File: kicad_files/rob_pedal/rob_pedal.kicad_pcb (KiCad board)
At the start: 2 copper layers, 56.5 x 56.8 mm, 52 parts, among them J1 OD_IN, J2 ODR_OUT, J3 9V, J4 SHO_IN, J5 SHO_OUT, Q1 BS170, Q2 BS170, Q3 BS170, Q4 BS170

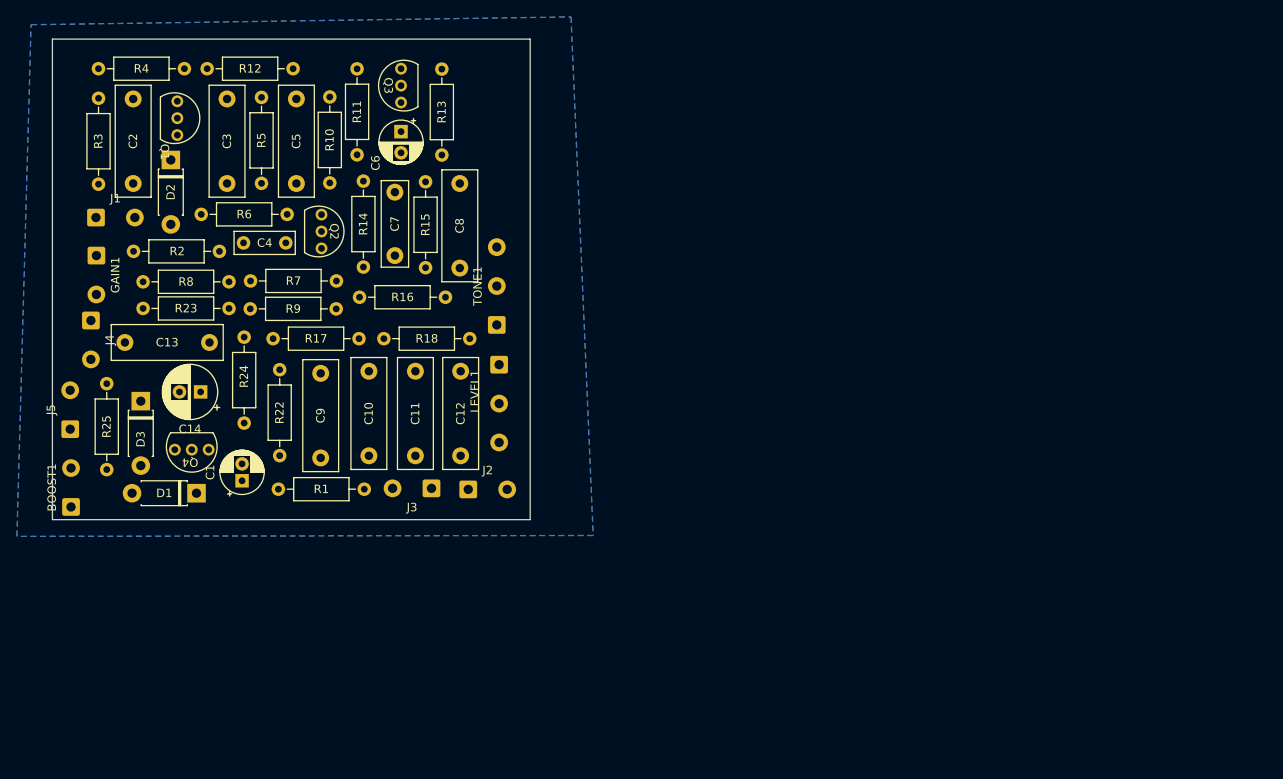
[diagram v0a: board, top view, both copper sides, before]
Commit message: added routing
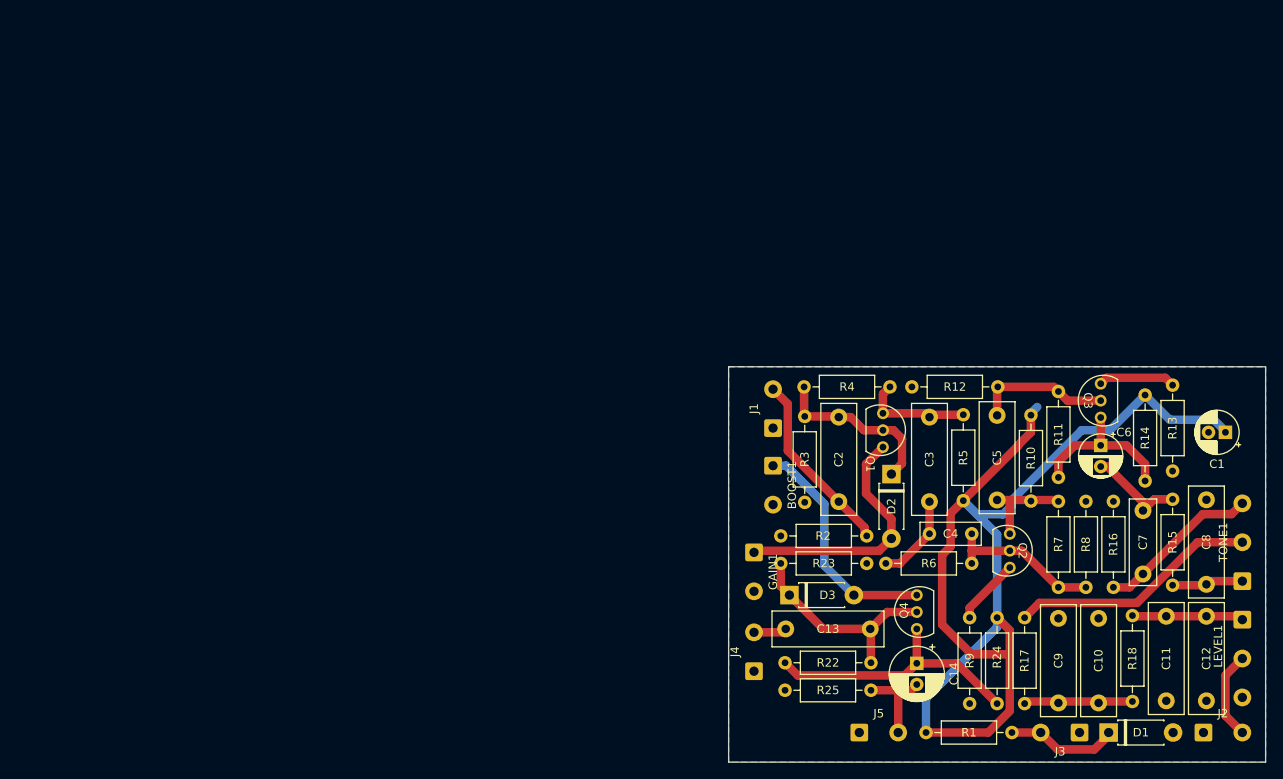
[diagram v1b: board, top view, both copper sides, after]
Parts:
- moved C1 116.4 mm to (184.3, 79.5), turned to 180 degrees
- moved R8 114.5 mm to (167.8, 87.7), turned to -90 degrees
- moved D1 111.5 mm to (170.5, 115.0), turned to 0 degrees
- moved R7 102.2 mm to (164.5, 97.8), turned to 90 degrees
- moved J5 100.0 mm to (141.0, 115.0), turned to 0 degrees
- moved R14 99.0 mm to (174.8, 85.2), turned to 90 degrees
- moved R18 98.4 mm to (173.3, 111.3), turned to 90 degrees
- moved R25 97.4 mm to (142.4, 110.0), turned to 180 degrees
- moved R9 97.0 mm to (154.0, 111.6), turned to 90 degrees
- moved C7 96.1 mm to (174.5, 88.8)
- moved R15 96.0 mm to (178.0, 87.4)
- moved C8 95.9 mm to (182.0, 97.5)
- moved R16 95.5 mm to (171.0, 97.8), turned to 90 degrees
- moved R24 95.0 mm to (157.3, 111.6)
- moved R17 94.8 mm to (160.5, 101.4), turned to -90 degrees
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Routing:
- net VCC: track 0.00 -> 134.8 mm
- net Net-(C14-Pad1): track 0.00 -> 32.3 mm
- net Net-(D2-Pad2): track 0.00 -> 29.8 mm
- net Net-(R17-Pad1): track 0.00 -> 29.4 mm
- net Net-(BOOST1-Pad1): track 0.00 -> 27.6 mm
- net Net-(C13-Pad2): track 0.00 -> 25.8 mm
- net ODR_IN: track 0.00 -> 21.3 mm
- net Net-(C2-Pad2): track 0.00 -> 20.8 mm
- net Net-(C7-Pad2): track 0.00 -> 19.4 mm
- net Net-(C6-Pad1): track 0.00 -> 19.1 mm
- net Net-(C4-Pad2): track 0.00 -> 18.8 mm
- net IN3: track 0.00 -> 16.3 mm
- net 9V: track 0.00 -> 13.3 mm
- net Net-(C3-Pad1): track 0.00 -> 13.3 mm
- net Net-(C11-Pad2): track 0.00 -> 13.2 mm
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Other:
- board size 56.5 x 56.8 mm -> 63.5 x 46.8 mm
